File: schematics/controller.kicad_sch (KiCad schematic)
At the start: 29 parts, among them IC1 AZ1117CD-3.3TRG1, IC2 ESP32-SOLO-1, J1 Conn_01x05, J2 Conn_01x05, J3 Conn_01x06, Q1 SS8050-G, Q2 SS8050-G, SW1 SW_Push, SW2 SW_Push, SW3 SW_Push_Dual, SW4 SW_Push_Dual, SW5 SW_Push_Dual, SW6 SW_Push_Dual, SW7 SW_Push_Dual

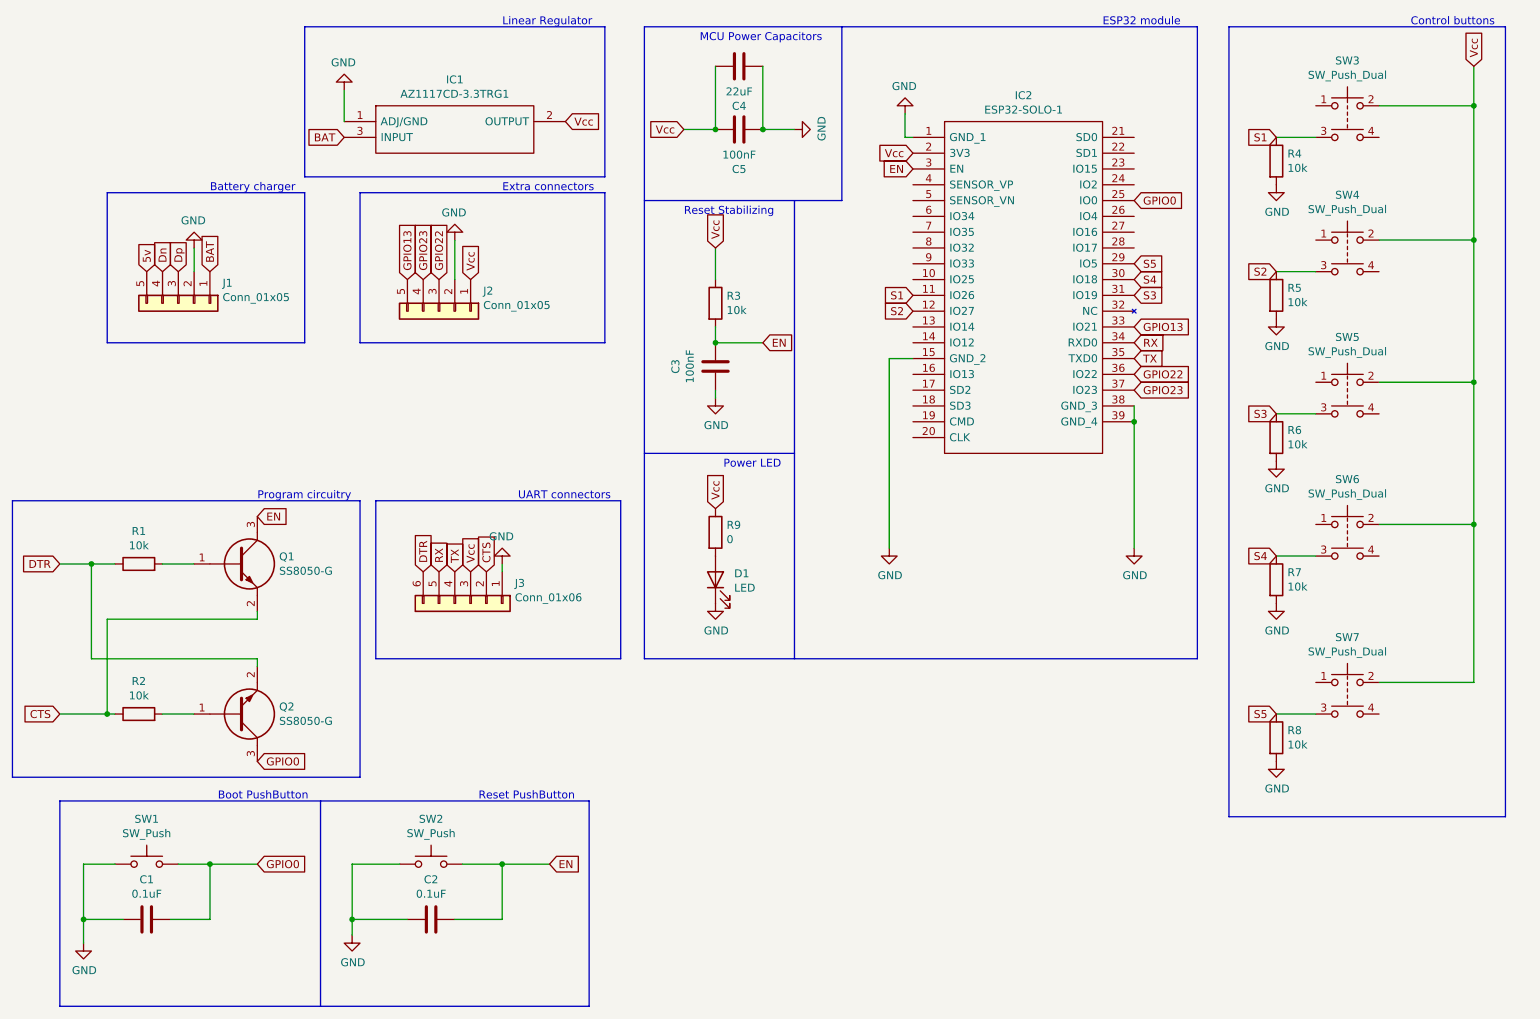
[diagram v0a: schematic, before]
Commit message: think Ive finished the schematics
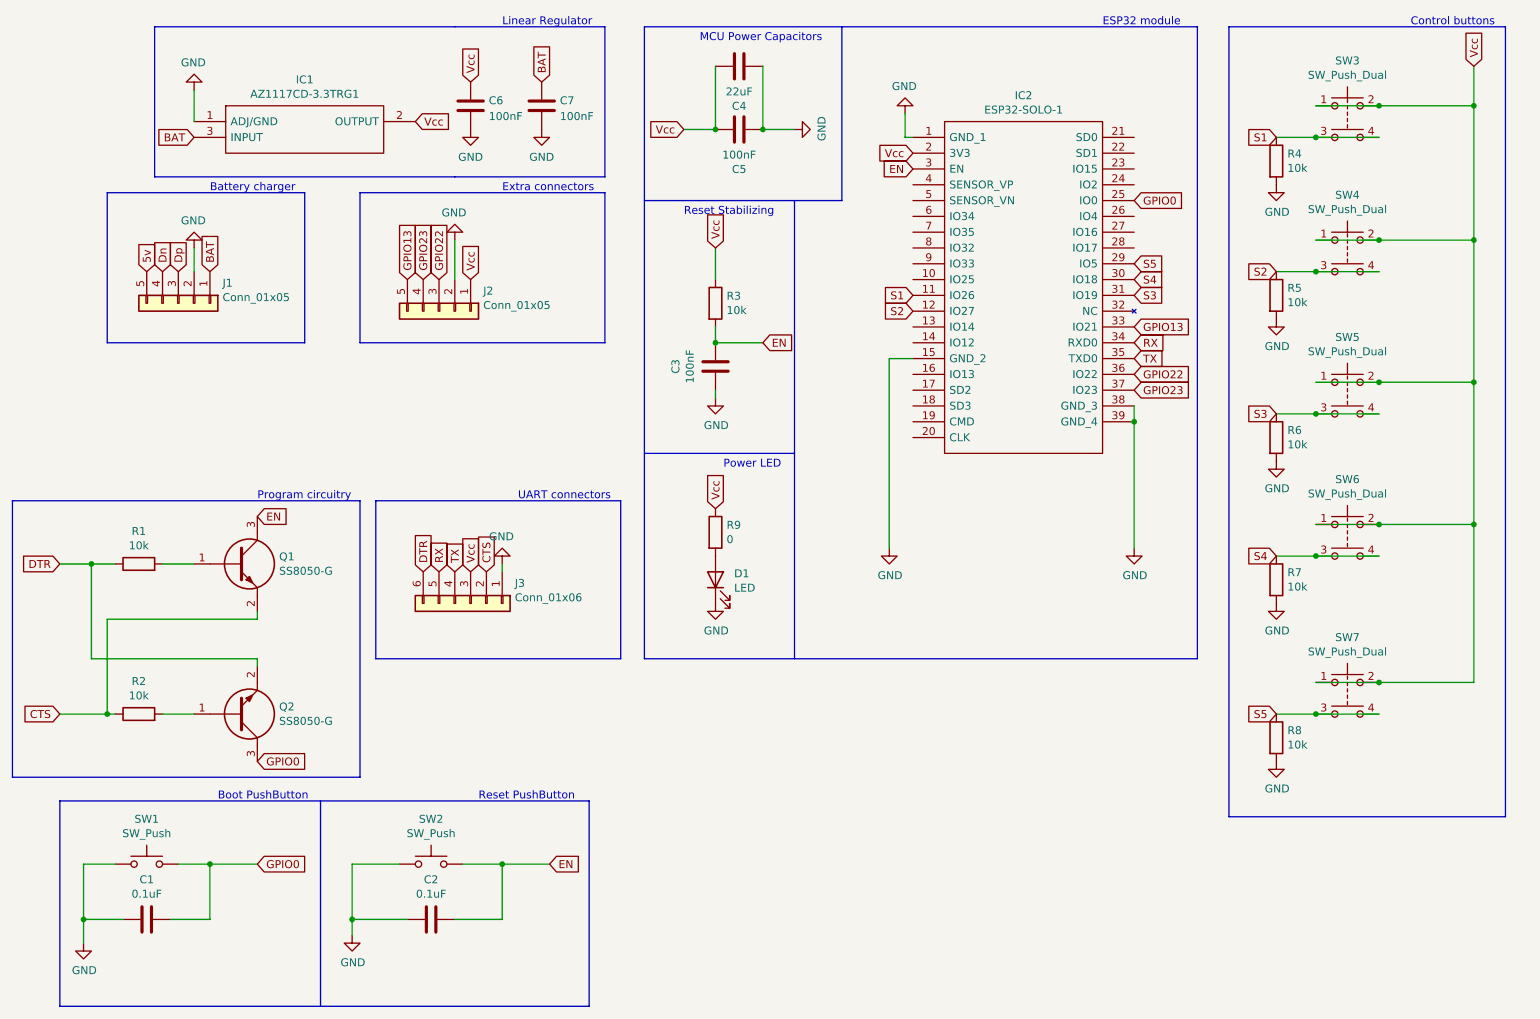
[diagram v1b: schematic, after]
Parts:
- added C6, C7: 100nF, Capacitor_SMD:C_0805_2012Metric, symbol Device:C
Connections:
- net BAT: now also C7.1
- net GND: now also C6.2, C7.2
- net S1: now also SW3.4
- net S2: now also SW4.4
- net S3: now also SW5.4
- net S4: now also SW6.4
- net S5: now also SW7.4
- net Vcc: now also SW3.1, SW4.1, SW5.1, SW6.1, SW7.1, C6.1
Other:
- moved on the sheet: IC1

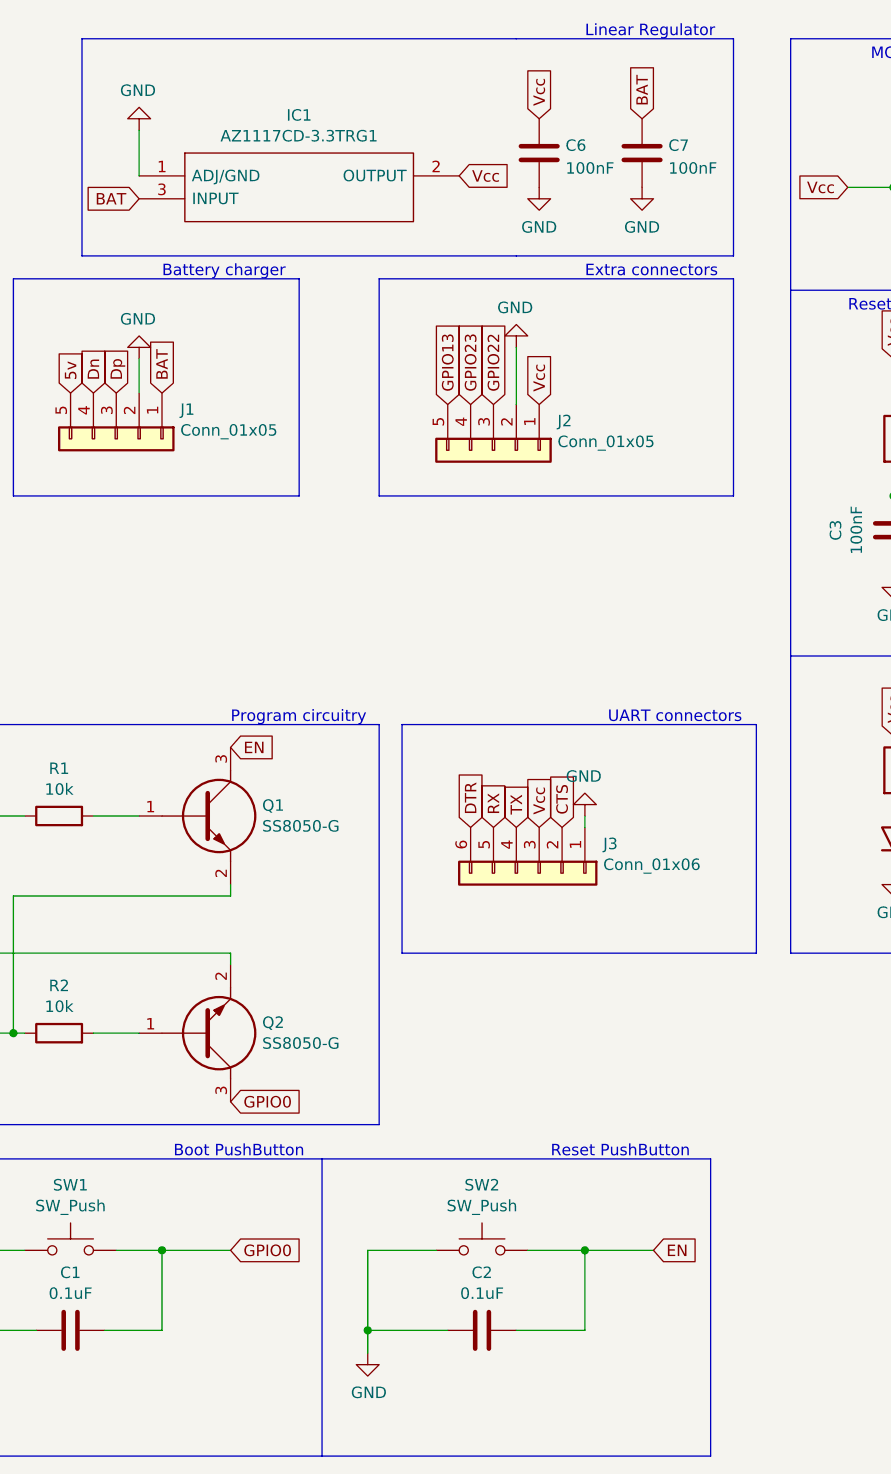
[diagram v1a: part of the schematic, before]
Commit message: final pcbs and schematics
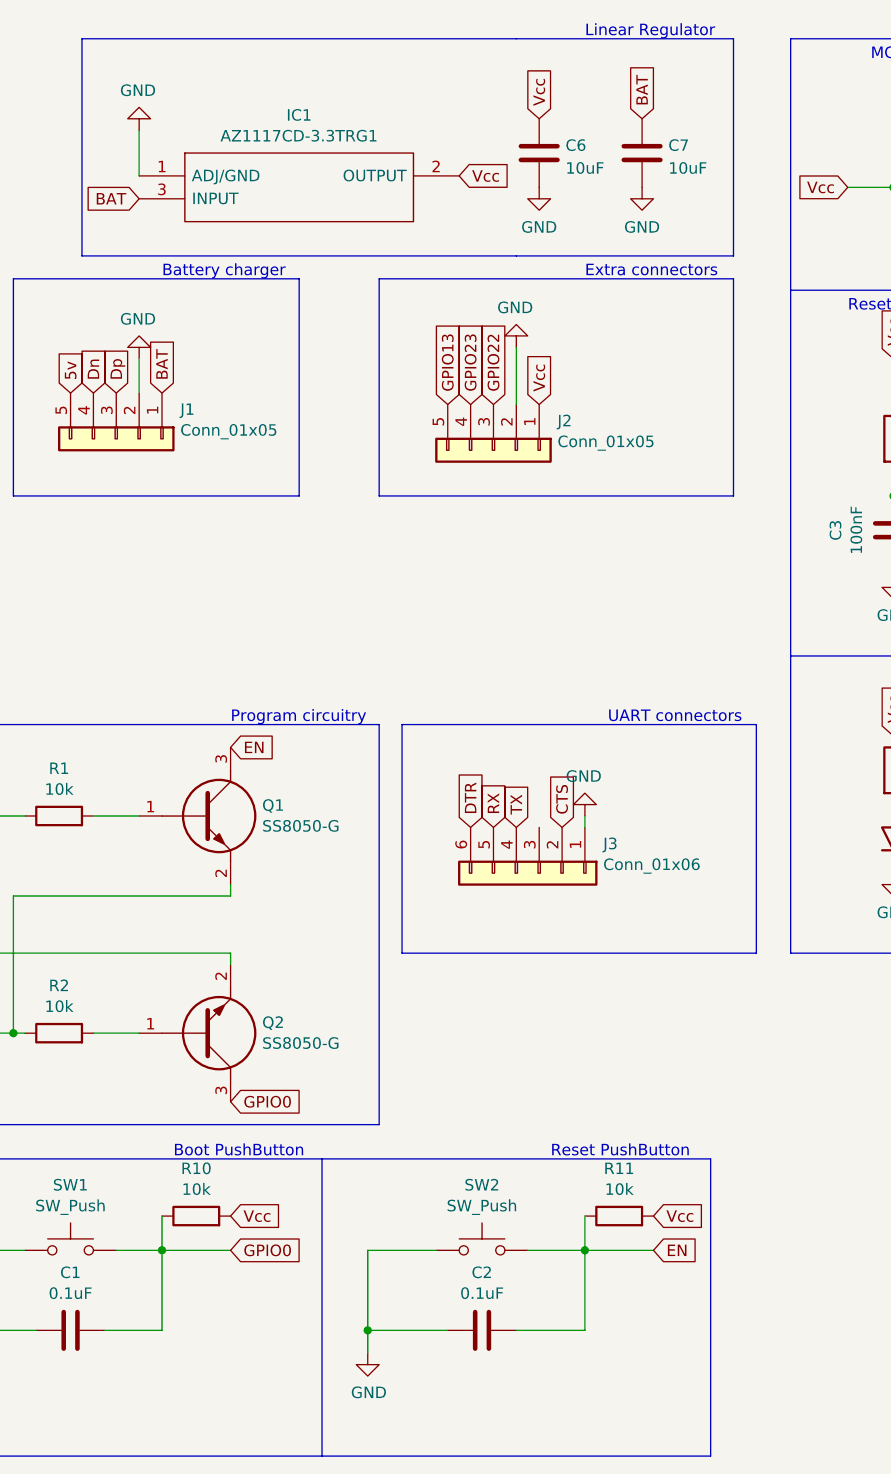
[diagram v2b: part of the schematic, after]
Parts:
- added R10, R11: 10k, Resistor_SMD:R_0805_2012Metric, symbol Device:R
- C6, C7: value 100nF -> 10uF
- IC2: footprint Mouser:ESP32SOLO1 -> RF_Module:ESP32-WROOM-32
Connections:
- net EN: now also R11.1
- net GPIO0: now also R10.1
- net Vcc: now also R10.2, R11.2; no longer J3.3 (Pin_3)
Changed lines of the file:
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@@
     (stroke (width 0) (type default) (color 0 0 0 0))
   )
-  (wire (pts (xy 57.15 161.29) (xy 57.15 152.4))
+  (wire (pts (xy 57.15 152.4) (xy 57.15 161.29))
     (stroke (width 0) (type default) (color 0 0 0 0))
   )
@@
     (stroke (width 0) (type default) (color 0 0 0 0))
   )
+  (wire (pts (xy 57.15 148.59) (xy 57.15 152.4))
+    (stroke (width 0) (type default) (color 0 0 0 0))
+  )
   (polyline (pts (xy 81.28 138.43) (xy 25.4 138.43))
     (stroke (width 0) (type default) (color 0 0 0 0))
@@
   )
   (wire (pts (xy 38.1 104.14) (xy 41.91 104.14))
+    (stroke (width 0) (type default) (color 0 0 0 0))
+  )
+  (wire (pts (xy 104.14 148.59) (xy 104.14 152.4))
     (stroke (width 0) (type default) (color 0 0 0 0))
   )
@@
     )
   )
+  (global_label "Vcc" (shape input) (at 111.76 148.59 0) (fields_autoplaced)
+    (effects (font (size 1.27 1.27)) (justify left))
+    (property "Intersheet References" "${INTERSHEET_REFS}" (id 0) (at 207.01 10.16 0)
+      (effects (font (size 1.27 1.27)) hide)
+    )
+  )
   (global_label "BAT" (shape input) (at 57.15 57.15 90) (fields_autoplaced)
     (effects (font (size 1.27 1.27)) (justify left))
@@
     )
   )
-  (global_label "Vcc" (shape input) (at 99.06 105.41 90) (fields_autoplaced)
-    (effects (font (size 1.27 1.27)) (justify left))
-    (property "Intersheet References" "${INTERSHEET_REFS}" (id 0) (at 0 0 0)
-      (effects (font (size 1.27 1.27)) hide)
-    )
-  )
   (global_label "Vcc" (shape input) (at 260.35 24.13 90) (fields_autoplaced)
     (effects (font (size 1.27 1.27)) (justify left))
@@
     (effects (font (size 1.27 1.27)) (justify right))
     (property "Intersheet References" "${INTERSHEET_REFS}" (id 0) (at 0 0 0)
+      (effects (font (size 1.27 1.27)) hide)
+    )
+  )
+  (global_label "Vcc" (shape input) (at 64.77 148.59 0) (fields_autoplaced)
+    (effects (font (size 1.27 1.27)) (justify left))
+    (property "Intersheet References" "${INTERSHEET_REFS}" (id 0) (at 160.02 10.16 0)
       (effects (font (size 1.27 1.27)) hide)
     )
@@
     (property "Reference" "IC2" (id 0) (at 187.96 28.829 0))
     (property "Value" "ESP32-SOLO-1" (id 1) (at 187.96 31.1404 0))
-    (property "Footprint" "Mouser:ESP32SOLO1" (id 2) (at 201.93 33.02 0)
+    (property "Footprint" "RF_Module:ESP32-WROOM-32" (id 2) (at 201.93 33.02 0)
       (effects (font (size 1.27 1.27)) (justify left) hide)
     )
@@
       (effects (font (size 1.27 1.27)) (justify left))
     )
-    (property "Value" "100nF" (id 1) (at 101.981 32.1822 0)
+    (property "Value" "10uF" (id 1) (at 101.981 32.1822 0)
       (effects (font (size 1.27 1.27)) (justify left))
     )
@@
     )
     (property "Datasheet" "~" (id 3) (at 99.06 30.48 0)
+      (effects (font (size 1.27 1.27)) hide)
+    )
+    (pin "1")
+    (pin "2")
+  )
+  (symbol (lib_id "Device:R") (at 107.95 148.59 90) (unit 1)
+    (in_bom yes) (on_board yes)
+    (property "Reference" "R11" (id 0) (at 107.95 143.3322 90))
+    (property "Value" "10k" (id 1) (at 107.95 145.6436 90))
+    (property "Footprint" "Resistor_SMD:R_0805_2012Metric" (id 2) (at 107.95 150.368 90)
+      (effects (font (size 1.27 1.27)) hide)
+    )
+    (property "Datasheet" "~" (id 3) (at 107.95 148.59 0)
       (effects (font (size 1.27 1.27)) hide)
     )
@@
       (effects (font (size 1.27 1.27)) (justify left))
     )
-    (property "Value" "100nF" (id 1) (at 113.411 32.1822 0)
+    (property "Value" "10uF" (id 1) (at 113.411 32.1822 0)
       (effects (font (size 1.27 1.27)) (justify left))
     )
@@
     (pin "1")
   )
+  (symbol (lib_id "Device:R") (at 60.96 148.59 90) (unit 1)
+    (in_bom yes) (on_board yes)
+    (property "Reference" "R10" (id 0) (at 60.96 143.3322 90))
+    (property "Value" "10k" (id 1) (at 60.96 145.6436 90))
+    (property "Footprint" "Resistor_SMD:R_0805_2012Metric" (id 2) (at 60.96 150.368 90)
+      (effects (font (size 1.27 1.27)) hide)
+    )
+    (property "Datasheet" "~" (id 3) (at 60.96 148.59 0)
+      (effects (font (size 1.27 1.27)) hide)
+    )
+    (pin "1")
+    (pin "2")
+  )
   (symbol (lib_id "power:GND") (at 110.49 34.29 0) (unit 1)
     (in_bom yes) (on_board yes) (fields_autoplaced)
@@
     )
     (path "/07a50c73-f63e-4cf3-a97f-e54f318e362e"
-      (reference "C6") (unit 1) (value "100nF") (footprint "Capacitor_SMD:C_0805_2012Metric")
+      (reference "C6") (unit 1) (value "10uF") (footprint "Capacitor_SMD:C_0805_2012Metric")
     )
     (path "/7015908c-1a2e-44bd-9cda-279b633533f3"
-      (reference "C7") (unit 1) (value "100nF") (footprint "Capacitor_SMD:C_0805_2012Metric")
+      (reference "C7") (unit 1) (value "10uF") (footprint "Capacitor_SMD:C_0805_2012Metric")
     )
     (path "/00000000-0000-0000-0000-00006226620c"
@@
     )
     (path "/00000000-0000-0000-0000-0000621e7cd6"
-      (reference "IC2") (unit 1) (value "ESP32-SOLO-1") (footprint "Mouser:ESP32SOLO1")
+      (reference "IC2") (unit 1) (value "ESP32-SOLO-1") (footprint "RF_Module:ESP32-WROOM-32")
     )
     (path "/00000000-0000-0000-0000-000062217fe3"
@@
       (reference "R9") (unit 1) (value "0") (footprint "Resistor_SMD:R_0805_2012Metric")
     )
+    (path "/c46700cb-8650-4446-aae2-40ac13fc1170"
+      (reference "R10") (unit 1) (value "10k") (footprint "Resistor_SMD:R_0805_2012Metric")
+    )
+    (path "/55a9d6d3-00cb-4662-99ba-03199a80f1ce"
+      (reference "R11") (unit 1) (value "10k") (footprint "Resistor_SMD:R_0805_2012Metric")
+    )
     (path "/00000000-0000-0000-0000-00006220c472"
